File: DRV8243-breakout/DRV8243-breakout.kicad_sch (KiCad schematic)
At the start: 27 parts, among them J1 Vin, J2 Motor_Output, J3 Conn_01x11_Pin, J4 Motor_Output, Q1 PMOS-AOD409, U1 PDRV8243HRXYQ1, U2 PDRV8243HRXYQ1

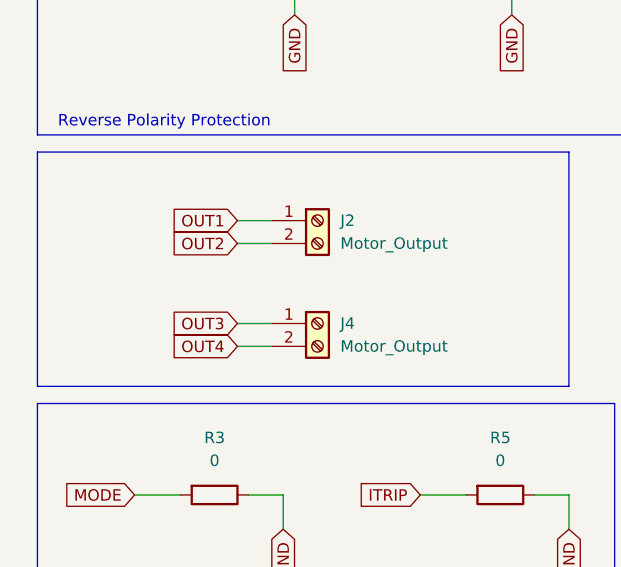
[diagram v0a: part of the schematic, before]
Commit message: Some more routing
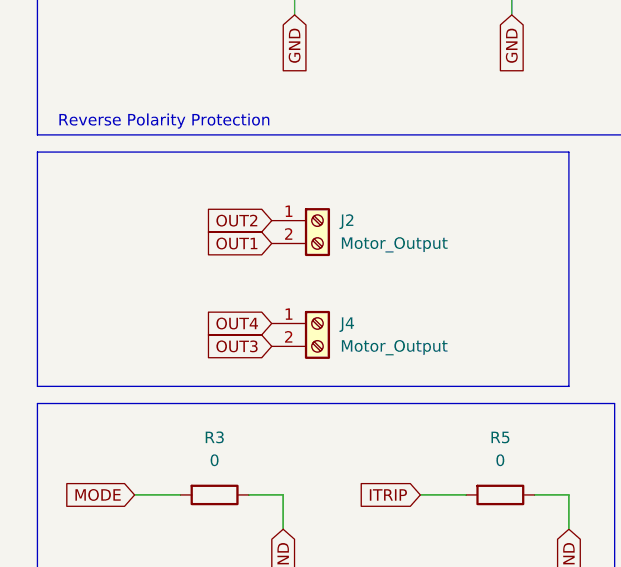
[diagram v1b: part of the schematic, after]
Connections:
- net OUT1: now also J2.2 (Pin_2); no longer J2.1 (Pin_1)
- net OUT2: now also J2.1 (Pin_1); no longer J2.2 (Pin_2)
- net OUT3: now also J4.2 (Pin_2); no longer J4.1 (Pin_1)
- net OUT4: now also J4.1 (Pin_1); no longer J4.2 (Pin_2)
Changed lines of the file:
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@@
-	(wire
-		(pts
-			(xy 41.91 85.09) (xy 45.72 85.09)
-		)
-		(stroke
-			(width 0)
-			(type default)
-		)
-	)
 	(wire
 		(pts
@@
 	(wire
 		(pts
-			(xy 41.91 93.98) (xy 45.72 93.98)
-		)
-		(stroke
-			(width 0)
-			(type default)
-		)
-	)
-	(wire
-		(pts
 			(xy 167.64 43.18) (xy 168.91 43.18)
 		)
@@
 	(wire
 		(pts
-			(xy 41.91 96.52) (xy 45.72 96.52)
-		)
-		(stroke
-			(width 0)
-			(type default)
-		)
-	)
-	(wire
-		(pts
 			(xy 63.5 160.02) (xy 63.5 161.29)
 		)
@@
 		(pts
 			(xy 226.06 53.34) (xy 237.49 53.34)
-		)
-		(stroke
-			(width 0)
-			(type default)
-		)
-	)
-	(wire
-		(pts
-			(xy 41.91 82.55) (xy 45.72 82.55)
 		)
 		(stroke
@@
 	(global_label "OUT1"
 		(shape input)
-		(at 41.91 82.55 180)
-		(fields_autoplaced yes)
-		(effects
-			(font
-				(size 1.27 1.27)
-			)
-			(justify right)
-		)
-		(property "Intersheetrefs" "${INTERSHEET_REFS}"
-			(at 34.0867 82.55 0)
+		(at 45.72 85.09 180)
+		(fields_autoplaced yes)
+		(effects
+			(font
+				(size 1.27 1.27)
+			)
+			(justify right)
+		)
+		(property "Intersheetrefs" "${INTERSHEET_REFS}"
+			(at 37.8967 85.09 0)
 			(effects
 				(font
@@
 	(global_label "OUT3"
 		(shape input)
-		(at 41.91 93.98 180)
-		(fields_autoplaced yes)
-		(effects
-			(font
-				(size 1.27 1.27)
-			)
-			(justify right)
-		)
-		(property "Intersheetrefs" "${INTERSHEET_REFS}"
-			(at 34.0867 93.98 0)
+		(at 45.72 96.52 180)
+		(fields_autoplaced yes)
+		(effects
+			(font
+				(size 1.27 1.27)
+			)
+			(justify right)
+		)
+		(property "Intersheetrefs" "${INTERSHEET_REFS}"
+			(at 37.8967 96.52 0)
 			(effects
 				(font
@@
 	(global_label "OUT2"
 		(shape input)
-		(at 41.91 85.09 180)
-		(fields_autoplaced yes)
-		(effects
-			(font
-				(size 1.27 1.27)
-			)
-			(justify right)
-		)
-		(property "Intersheetrefs" "${INTERSHEET_REFS}"
-			(at 34.0867 85.09 0)
+		(at 45.72 82.55 180)
+		(fields_autoplaced yes)
+		(effects
+			(font
+				(size 1.27 1.27)
+			)
+			(justify right)
+		)
+		(property "Intersheetrefs" "${INTERSHEET_REFS}"
+			(at 37.8967 82.55 0)
 			(effects
 				(font
@@
 	(global_label "OUT4"
 		(shape input)
-		(at 41.91 96.52 180)
-		(fields_autoplaced yes)
-		(effects
-			(font
-				(size 1.27 1.27)
-			)
-			(justify right)
-		)
-		(property "Intersheetrefs" "${INTERSHEET_REFS}"
-			(at 34.0867 96.52 0)
-			(effects
-				(font
+		(at 45.72 93.98 180)
+		(fields_autoplaced yes)
+		(effects
+			(font
+				(size 1.27 1.27)
+			)
+			(justify right)
+		)
+		(property "Intersheetrefs" "${INTERSHEET_REFS}"
+			(at 37.8967 93.98 0)
+			(effects
+				(font
